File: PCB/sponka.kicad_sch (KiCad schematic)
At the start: 9 parts, among them J1 Conn_01x03_Pin, J4 Conn_01x05_Pin, SW1 SW_Push, U1 CH32V003FxUx

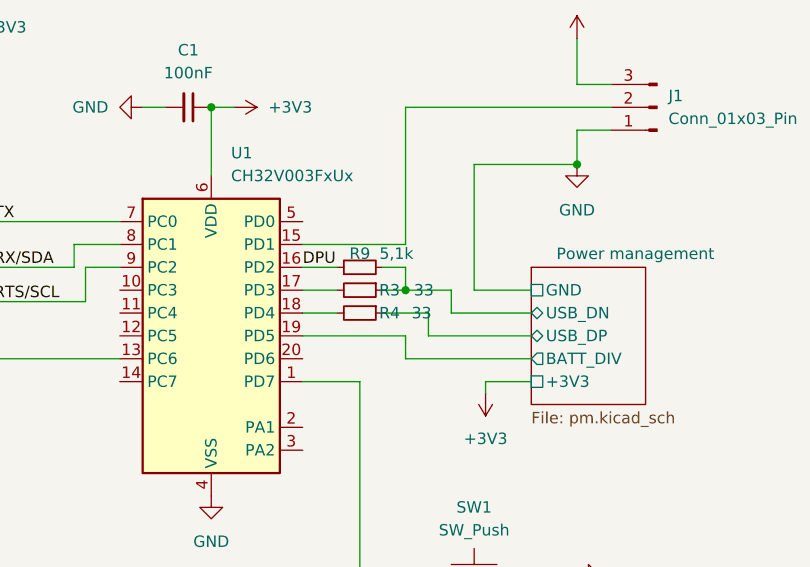
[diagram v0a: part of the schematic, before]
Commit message: Fix wrong values
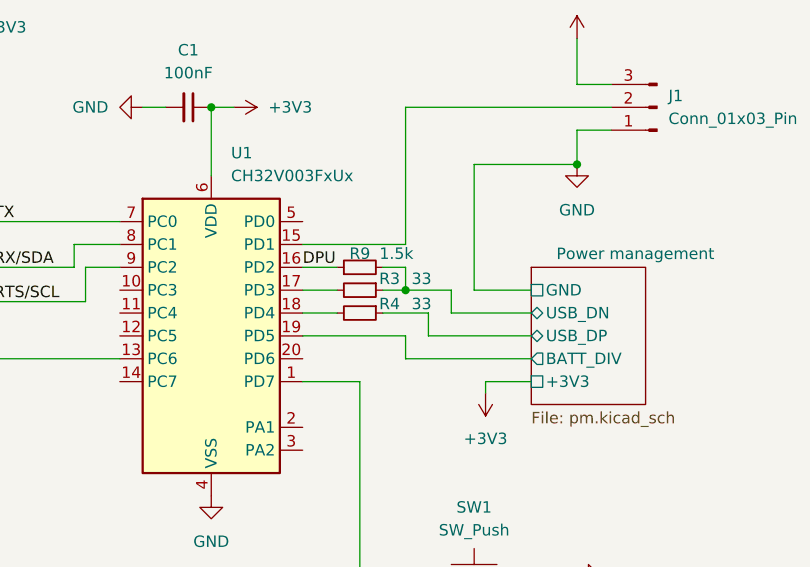
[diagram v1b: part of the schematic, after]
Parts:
- R9: value 5,1k -> 1.5k
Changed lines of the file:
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@@
 			)
 		)
-		(property "Value" "5,1k"
+		(property "Value" "1.5k"
 			(at 165.354 81.026 90)
 			(effects
@@
 		(dnp no)
 		(property "Reference" "R3"
-			(at 164.592 85.09 90)
+			(at 164.592 83.82 90)
 			(effects
 				(font
@@
 		)
 		(property "Value" "33"
-			(at 168.402 85.09 90)
+			(at 168.148 83.82 90)
 			(effects
 				(font
@@
 		(dnp no)
 		(property "Reference" "R4"
-			(at 164.592 87.63 90)
+			(at 164.592 86.614 90)
 			(effects
 				(font
@@
 		)
 		(property "Value" "33"
-			(at 168.148 87.63 90)
-			(effects
-				(font
+			(at 168.148 86.614 90)
+			(effects
+				(font
